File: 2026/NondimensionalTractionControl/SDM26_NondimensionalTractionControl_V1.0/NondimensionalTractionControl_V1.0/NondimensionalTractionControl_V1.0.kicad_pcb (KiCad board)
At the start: 4 copper layers, 70 x 35 mm, 61 parts, among them IC1 STM32H743VIT6, IC2 74LVC1G17SE-7, IC3 TLP175A_TPL,E, IC4 SN65HVD230QDR, IC5 TPS259250DRCR, IC6 MIC37100-3.3WS, IC7 TPS2116DRLR, J1 104031-0811, J2 Conn_ARM_SWD_TagConnect_TC203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, J3 USB_B_Micro, J4 SM04B-ULHK-1TA1-ETB_HF_, J5 SM04B-ULHK-1TA1-ETB_HF_, J6 SM04B-ULHK-1TA1-ETB_HF_, U1 USBLC6-2SC6, Y1 ABM3B-8.000MHZ-10-1-U-T

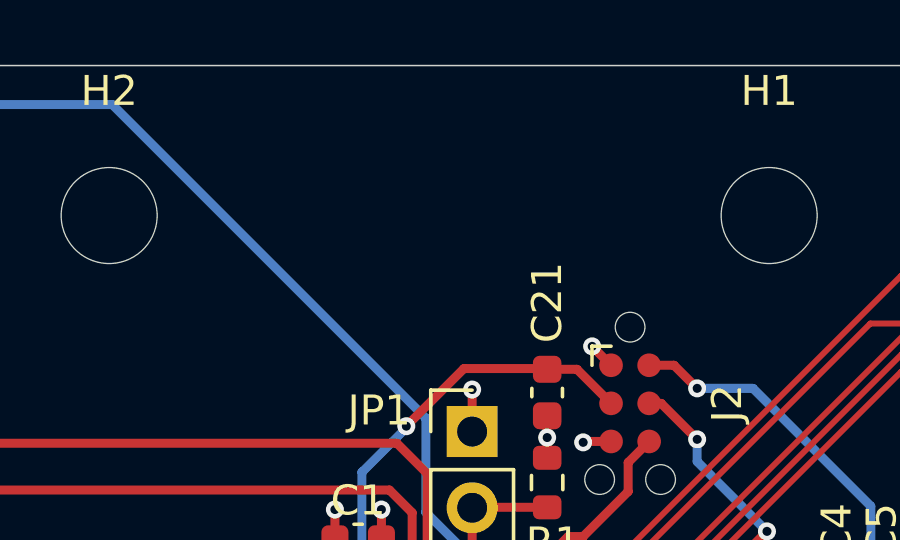
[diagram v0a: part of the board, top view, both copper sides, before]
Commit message: Final Final update for September order
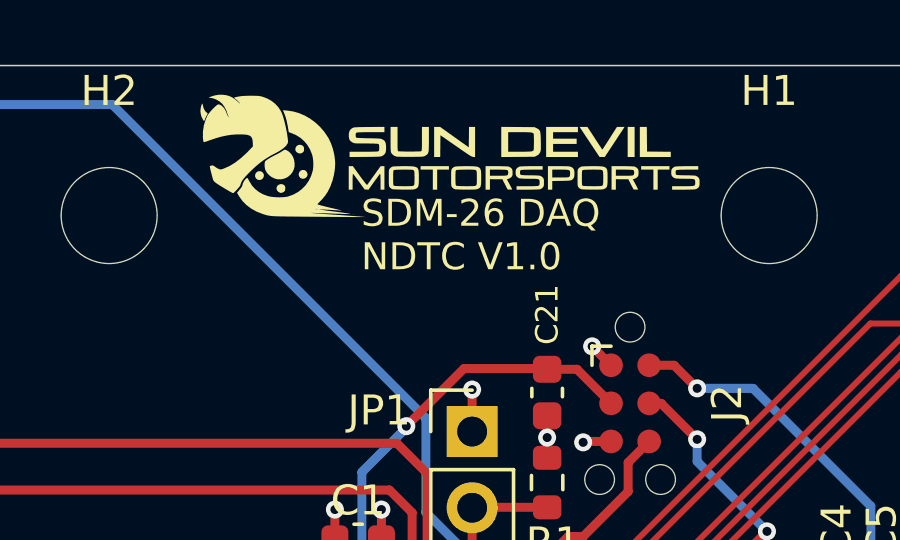
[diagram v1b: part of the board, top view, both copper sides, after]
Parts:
- added G***: LOGO, LOGO, F.Cu at (125.4, 118.0)
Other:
- board text added: "SDM-26 DAQ NDTC V1.0"
